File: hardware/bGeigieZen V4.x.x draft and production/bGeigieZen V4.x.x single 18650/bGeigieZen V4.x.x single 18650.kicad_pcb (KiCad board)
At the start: 2 copper layers, 129.4 x 64.6 mm, 13 parts, among them J1 M5 2x15 pin, J3 GPS, J4 Geiger Safepulse, J5 Extra support header, SW1 SW_SPDT

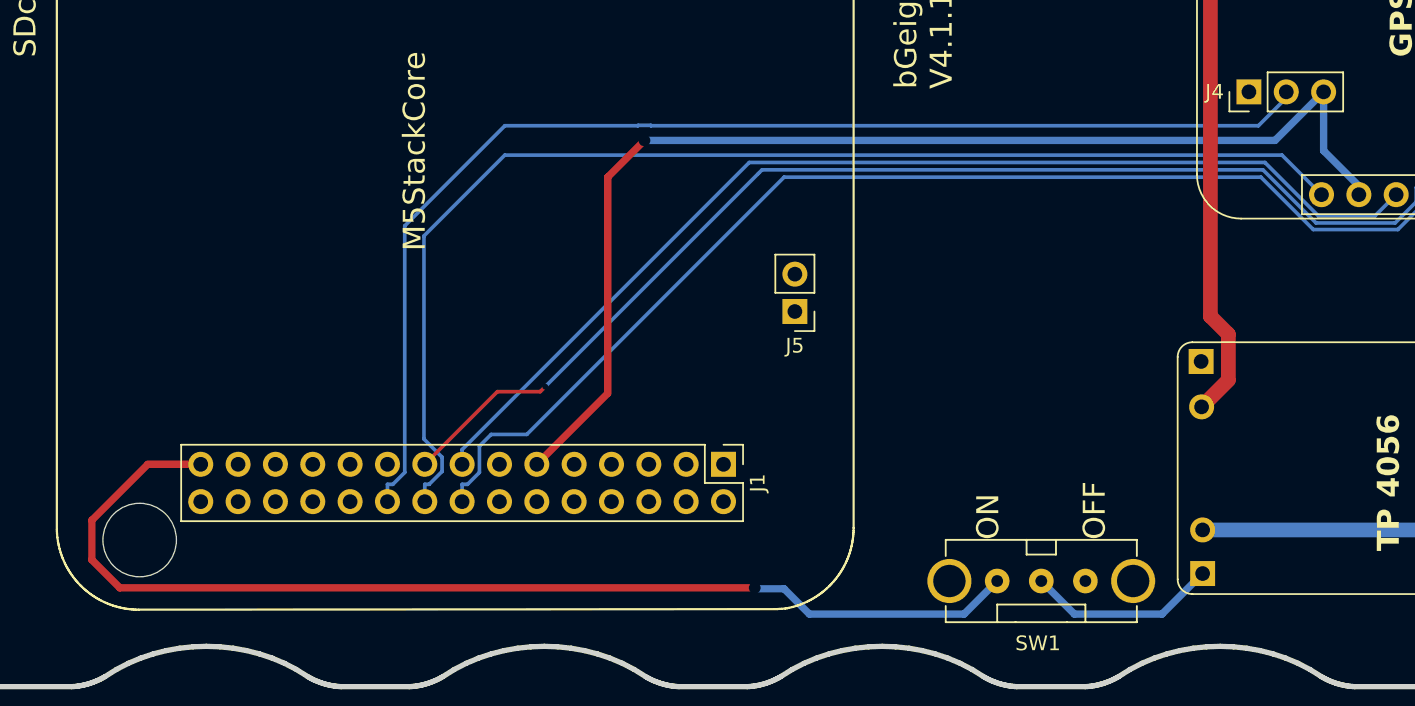
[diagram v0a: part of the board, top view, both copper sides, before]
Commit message: Board and files updated
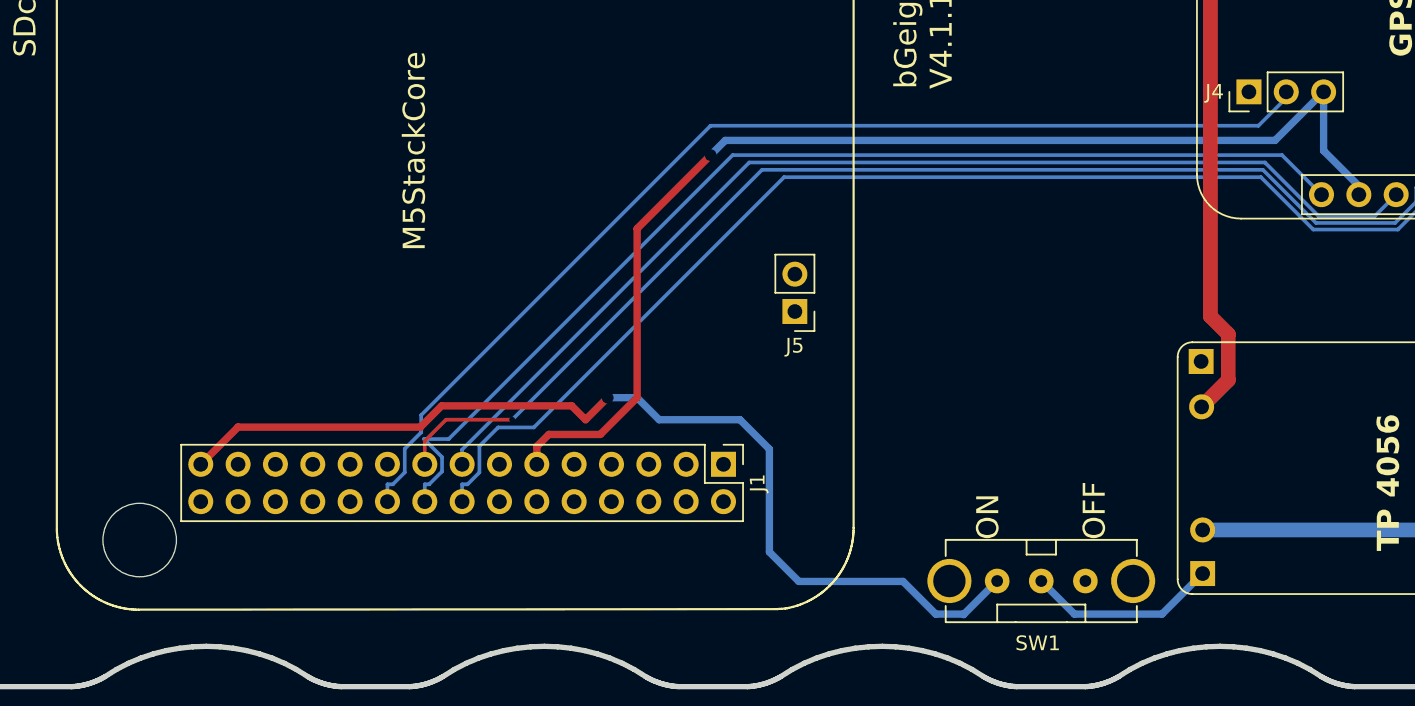
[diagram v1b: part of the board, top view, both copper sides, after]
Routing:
- net /GIO2 on Core and GIO32 on Core-2: track 83.5 -> 75.2 mm
- net /SCL: track 84.4 -> 76.4 mm
- net /BAT: track 75.7 -> 68.0 mm
- net 3.3V: track 80.6 -> 79.4 mm
- net /SDA: track 86.1 -> 87.0 mm
